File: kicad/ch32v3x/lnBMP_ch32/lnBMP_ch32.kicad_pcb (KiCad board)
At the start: 2 copper layers, 72.6 x 33 mm, 24 parts, among them J1 BMP Debug1, J2 BMP Debug2, J3 Debug port, J4 USB_OTG, SW1 SW_DIP_x01, SW2 SW_DIP_x01, U1 CH32V303RCT6, U2 LM1117-3.3, Y1 Crystal

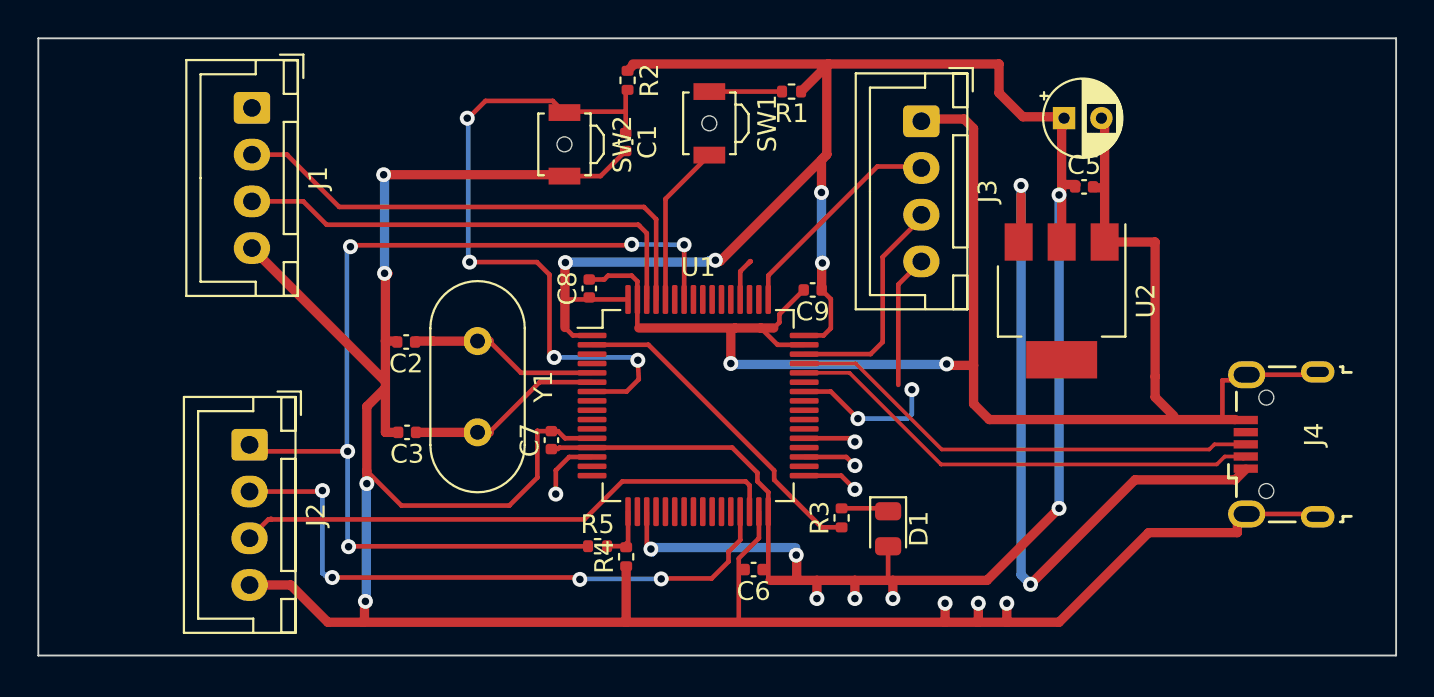
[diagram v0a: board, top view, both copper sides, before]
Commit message: kicad: minor update
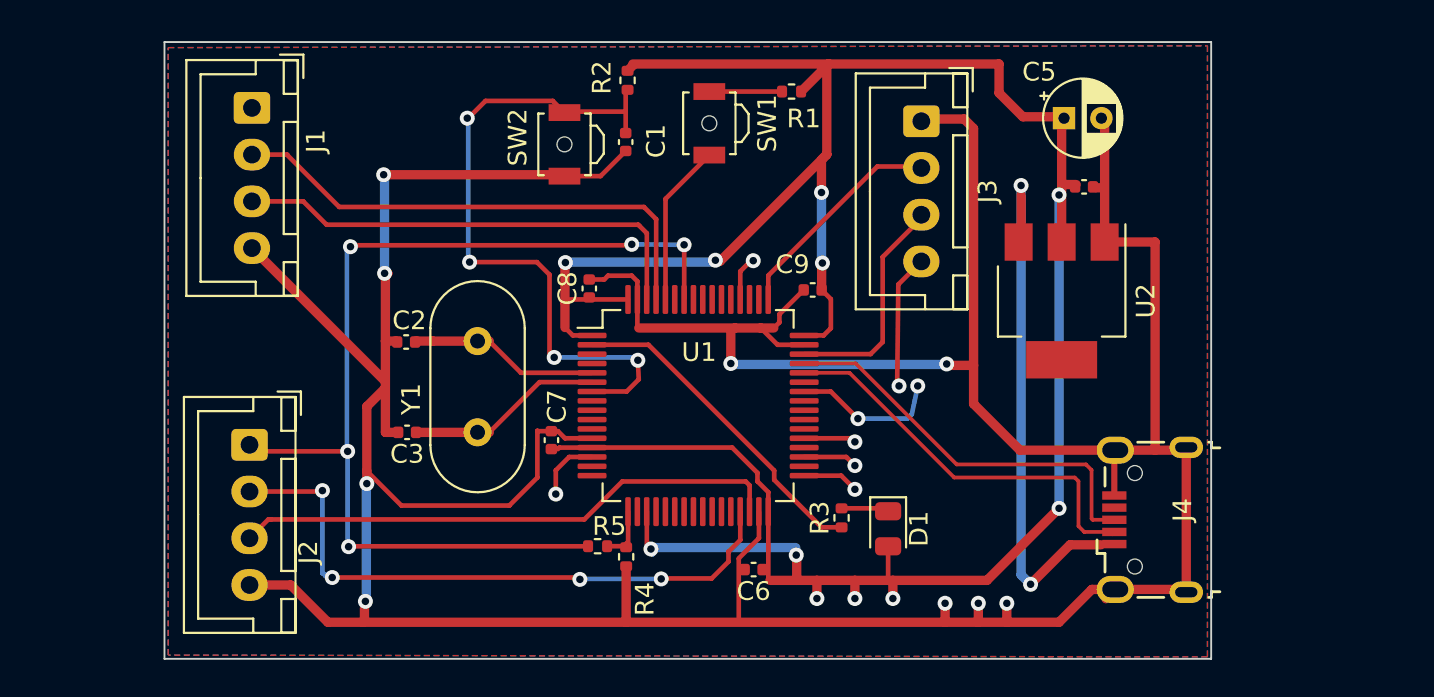
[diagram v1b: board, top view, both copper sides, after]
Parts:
- moved J4 8.11 mm to (154.7, 92.6)
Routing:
- net GND: track 236.4 -> 226.7 mm
- net Net-(J4-VBUS): track 38.0 -> 28.6 mm
- net D-: track 26.0 -> 21.7 mm
- net D+: track 25.6 -> 21.6 mm
- net unconnected-(U1-PC11-Pad52): track 2.46 -> 2.75 mm, vias 0 -> 1
- net UART TX: track 7.11 -> 7.28 mm, vias 0 -> 1
- added copper zone on B.Cu, net GND
- added copper zone on F.Cu, net GND
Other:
- board size 72.6 x 33 mm -> 56 x 33 mm
